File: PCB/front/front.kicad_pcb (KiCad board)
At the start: 2 copper layers, 43 x 26 mm, 22 parts, among them J1 Conn_01x06_Pin, J2 Conn_01x06_Pin, J3 Conn_01x08_Pin, U1 VL53L1CXV0FY1

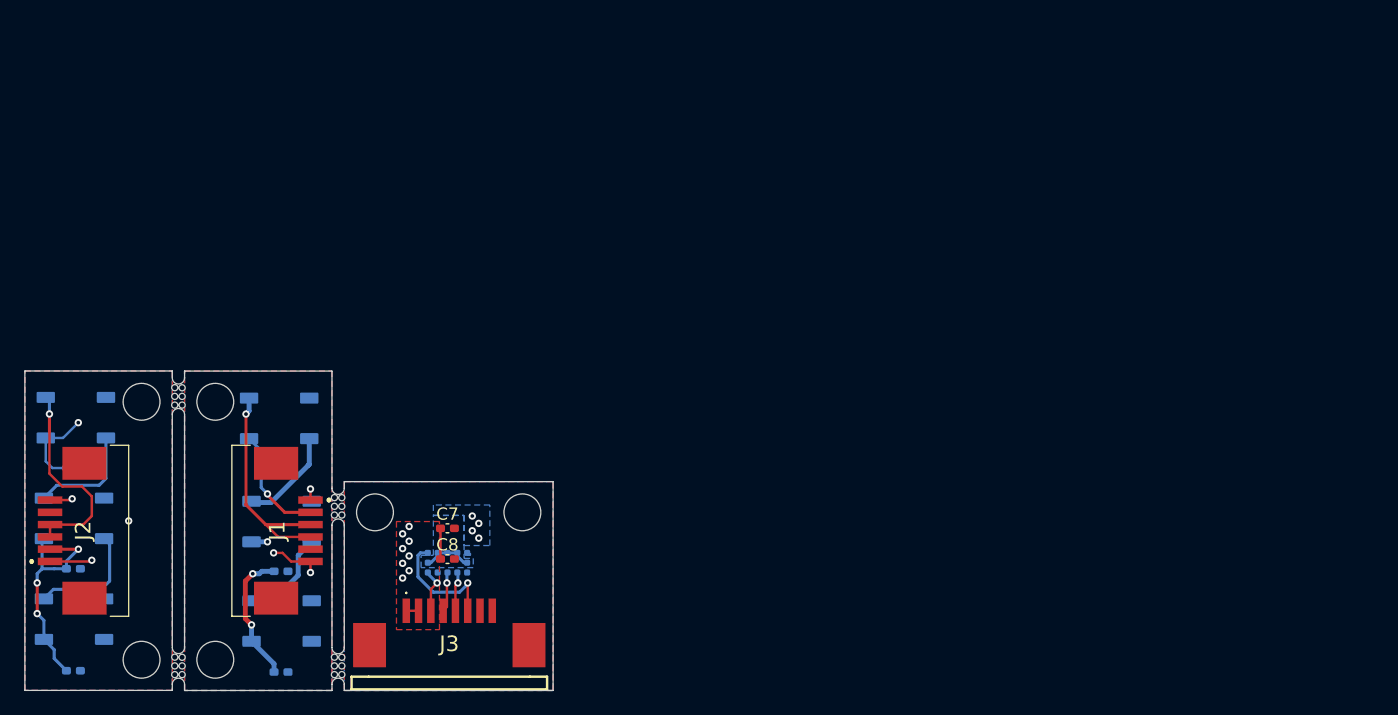
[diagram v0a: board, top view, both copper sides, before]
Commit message: random
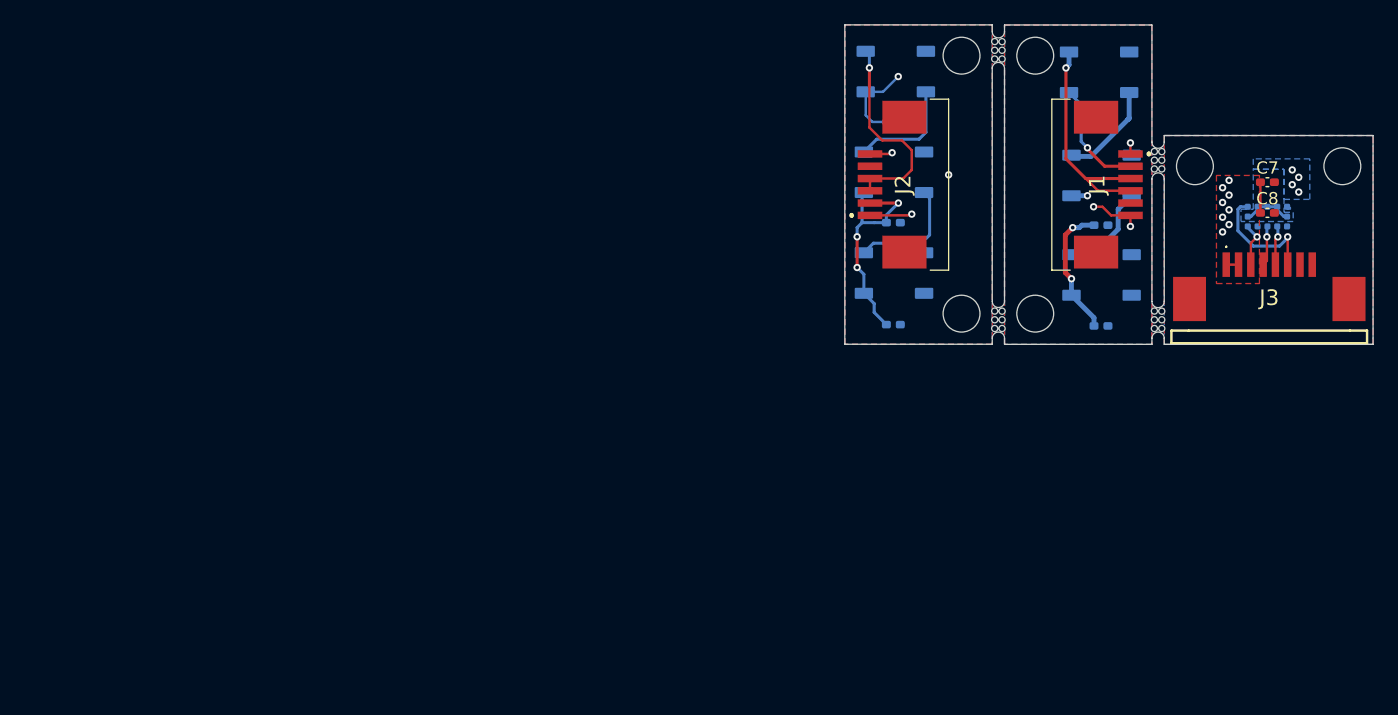
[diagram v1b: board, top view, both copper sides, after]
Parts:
- moved C2 72.5 mm to (143.3, 105.3)
- moved C3 72.5 mm to (143.3, 97.1)
- moved C7 72.5 mm to (156.9, 93.6)
- moved C8 72.5 mm to (156.9, 96.1)
- moved D2 72.5 mm to (143.4, 93.1)
- moved D3 72.5 mm to (143.4, 101.2)
- moved D4 72.5 mm to (126.6, 84.6)
- moved D6 72.5 mm to (126.5, 101.0)
- moved J3 72.5 mm to (157.0, 103.5)
- moved TP1 72.5 mm to (135.0, 82.9)
- moved TP2 72.5 mm to (135.0, 104.8)
- moved TP3 72.5 mm to (148.0, 104.8)
- moved TP4 72.5 mm to (148.0, 91.8)
- moved U1 72.5 mm to (156.9, 96.4)
- moved C1 72.5 mm to (143.3, 88.9)
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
